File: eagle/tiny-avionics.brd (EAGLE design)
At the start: 65.8 x 25.4 mm, 69 parts, among them IC1 BQ24022, J1 USB-MICROB, J3 JST-PH-2-SMT-RA, U1 LP5907, U2 M25P10-AVMN6TP_TR, U3 LSM9DS0, U5 LTC1998, U6 ATMEGA32U4-AU, X1 8MHz

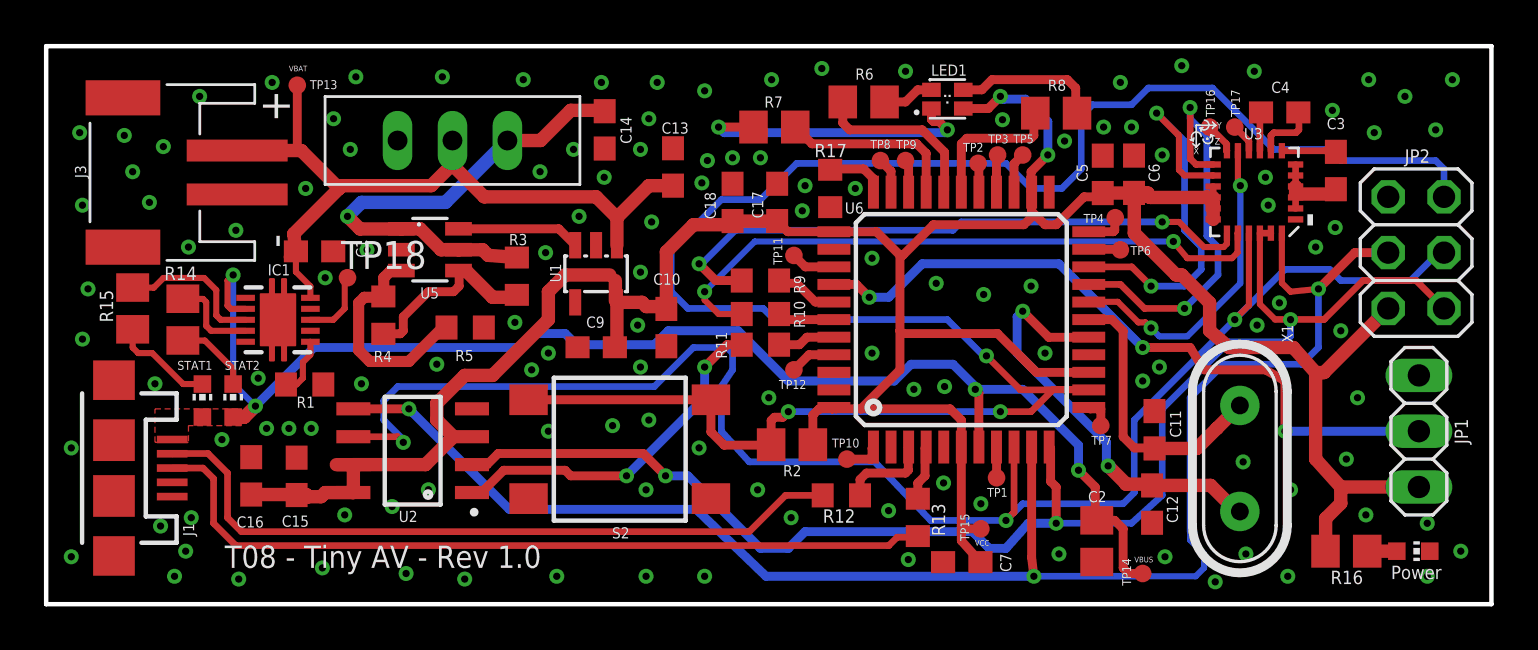
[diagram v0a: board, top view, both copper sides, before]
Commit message: Merge commit to overwrite eagle files
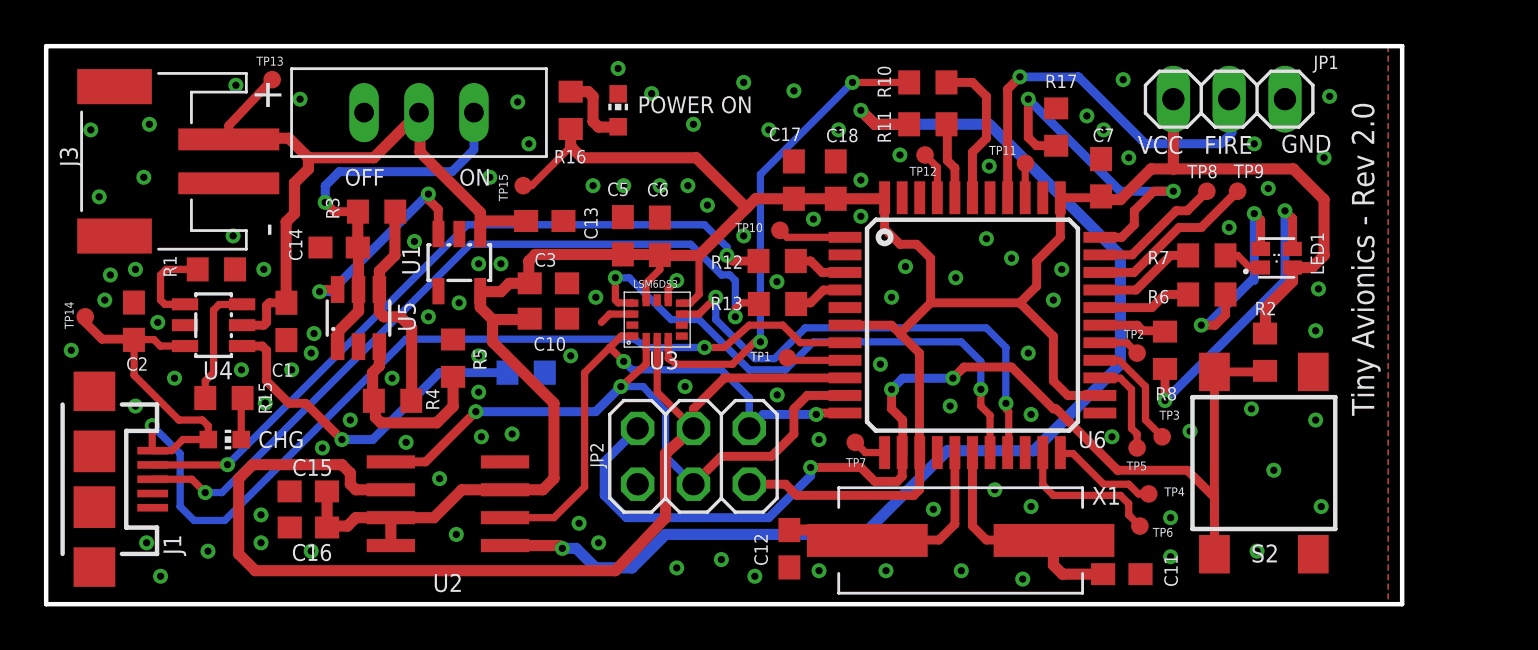
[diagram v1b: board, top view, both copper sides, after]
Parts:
- removed C4: .22µ, rcl:C0603
- removed C9: 2.2µ, rcl:C0603
- removed IC1: BQ24022, tinyav-lib:DRC-S-PVSON-N10
- removed LED3: (no value), adafruit:CHIP-LED0603
- removed R14: 330, rcl:R0805
- removed R9: 0, rcl:R0603
- removed TP16, TP17, TP18: TPTP08R, testpad:TP08R
- added U$1: 10k B25/50=3375k, tinyav-lib:R0603
- added U4: BQ21040, tinyav-lib:SOT23-6L
- C2: device rcl:C0805 -> rcl:C0603
- C3: value 4.7µ -> 2.2µ
- R1: value 4k -> 5.36k
- R15, R16, R6, R7, R8: value 330 -> 3.3k; device rcl:R0805 -> rcl:R0603
- R2: device rcl:R0805 -> rcl:R0603
- U2: value M25P10-AVMN6TP_TR -> M25PX16; device SOIC127P600X175-8N:SOIC127P600X175-8N -> tinyav-lib:SO8
- U3: value LSM9DS0 -> LSM6DS3; device LSM9DS0:LGA-24 -> tinyav-lib:LGA-14L
- X1: device IQD-Frequency-Products:HC49 -> tinyav-lib:ATS-SM
- moved TP14 49.5 mm to (1.78, 13.1)
- moved C2 45.0 mm to (4.00, 12.9), turned to 90 degrees
- moved LED4 41.4 mm to (26.0, 22.5), turned to 0 degrees
- moved R16 40.6 mm to (23.9, 22.5), turned to 270 degrees
- moved C3 36.2 mm to (22.9, 14.6), turned to 0 degrees
- moved JP2 34.2 mm to (29.5, 6.73), turned to 180 degrees
- moved S2 29.3 mm to (55.4, 6.42), turned to 270 degrees
- moved U3 27.8 mm to (27.8, 13.0)
- moved TP15 26.0 mm to (21.7, 19.1)
- moved C5 22.0 mm to (26.2, 16.8)
- moved R2 21.9 mm to (55.5, 11.5), turned to 90 degrees
- moved C6 21.8 mm to (27.9, 16.7)
- moved R7 20.5 mm to (52.8, 15.9), turned to 0 degrees
- moved C7 18.6 mm to (48.0, 19.4), turned to 90 degrees
- moved R6 17.9 mm to (52.8, 14.1)
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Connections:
- net N$52 renamed TP3
- net N$54 renamed TP12
- net N$55 renamed TP11
- net N$56 renamed TP10
- net N$57 renamed TP9
- net N$58 renamed TP8
- net N$59 renamed TP7
- net N$60 renamed TP1
- net N$61 renamed TP2
- net N$62 renamed TP4
- net N$63 renamed TP5
- net N$64 renamed TP6
- removed net GYR_EN: R9.1, U3.19
- removed net N$16: U3.14, U6.20
- removed net N$17: U3.13, U6.19
- removed net N$19: U3.11, U6.18
- removed net N$20: R9.2, U6.38
- removed net N$50: IC1.3, R15.2
- removed net N$51: IC1.4, R14.2
- removed net N$66: TP17.TP, U3.10
- removed net N$67: TP16.TP, U3.12
- removed net N$68: IC1.8, TP18.TP
- net CLK: now also U3.13; no longer U3.21
- net GND: now also C3.2, U$1.2, U3.7, U4.5; no longer C3.1, C9.2, IC1.5, IC1.7, IC1.9, U3.4, U3.5
- net MISO: now also U3.1; no longer U3.22, U3.23
- net MOSI: now also U3.14; no longer U3.24
- net N$10: now also U3.4, U6.18; no longer C4.2, U3.8
- net N$11: now also U6.19; no longer C4.1
- net N$13: now also U4.2; no longer IC1.10
- net N$4: now also R15.2, U4.3; no longer IC1.6, R1.2
- net N$49: now also R1.2, U4.4; no longer LED3.C, R14.1
- net N$9: now also U$1.1, U4.1; no longer C3.2, U3.7
- net VBUS1: now also U4.6; no longer IC1.2, LED3.A
- net VCC: now also C3.1, U3.5, U3.8; no longer C9.1, U3.15, U3.16, U3.17, U3.18
- net XM_EN: now also U3.12; no longer U3.20
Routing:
- net MOSI: track 73.6 -> 30.2 mm, vias 3 -> 2
- net N$3: track 95.2 -> 54.2 mm
- net MISO: track 64.2 -> 25.6 mm, vias 3 -> 2
- net MEM_EN: track 16.1 -> 54.2 mm
- net GYR_EN: track 28.1 -> 0.00 mm, vias 2 -> 0
- net CLK: track 75.1 -> 49.9 mm, vias 3 -> 0
- net N$10: track 2.88 -> 25.4 mm, vias 0 -> 2
- net N$11: track 1.77 -> 22.6 mm, vias 0 -> 2
- net N$17: track 18.6 -> 0.00 mm, vias 2 -> 0
- net N$16: track 18.4 -> 0.00 mm, vias 2 -> 0
- net N$19: track 14.6 -> 0.00 mm, vias 2 -> 0
- net FIRE_EN: track 32.1 -> 18.4 mm, vias 3 -> 1
- net N$9: track 2.46 -> 15.9 mm, vias 0 -> 1
- net N$65: track 2.78 -> 16.1 mm, vias 0 -> 2
- net N$1: track 13.6 -> 1.83 mm, vias 2 -> 0
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- removed copper zone on layer 1, net VBUS1
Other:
- board size 65.8 x 25.4 mm -> 61.7 x 25.4 mm
- board text added: "CHG"
- board text added: "FIRE"
- board text added: "GND"
- board text added: "OFF"
- board text added: "ON"
- board text added: "POWER ON"
- board text added: "Tiny Avionics - Rev 2.0"
- board text removed: "Power"
- board text removed: "STAT1"
- board text removed: "STAT2"
- board text removed: "T08 - Tiny AV - Rev 1.0"
- board text removed: "VBAT"
- board text removed: "VBUS"
